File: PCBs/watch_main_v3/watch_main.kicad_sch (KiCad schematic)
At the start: 1 part, among them U101 Watch_Outline_V2

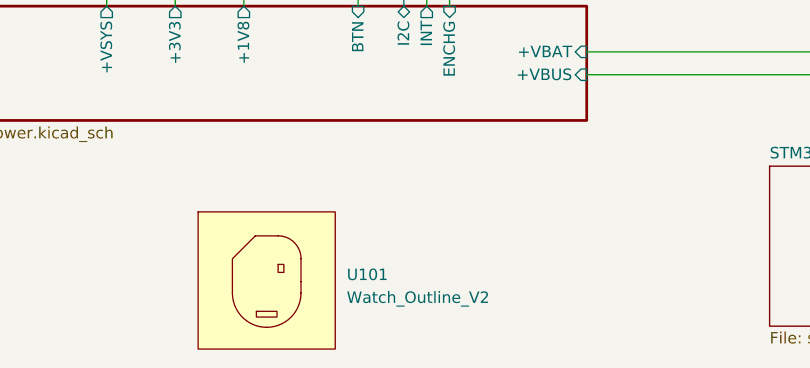
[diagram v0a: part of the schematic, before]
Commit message: watch_main_v3 updates
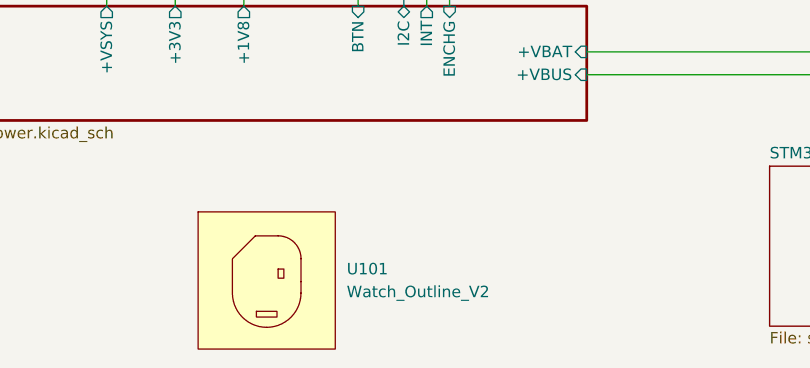
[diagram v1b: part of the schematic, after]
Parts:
- U101: footprint watch_footprints:Watch Outline V2 -> watch_footprints:Watch Outline V3; symbol watch_symbols_lib:Watch_Outline_V2 -> watch_symbols_lib:Watch_Outline_V3
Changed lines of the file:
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@@
     )
   )
-  (symbol (lib_id "watch_symbols_lib:Watch_Outline_V2") (at 73.66 177.8 0) (unit 1)
+  (symbol (lib_id "watch_symbols_lib:Watch_Outline_V3") (at 73.66 177.8 0) (unit 1)
     (in_bom no) (on_board yes) (dnp no) (fields_autoplaced)
-    (property "Reference" "U101" (at 82.55 177.165 0)
+    (property "Reference" "U101" (at 82.55 176.53 0)
       (effects (font (size 1.27 1.27)) (justify left))
     )
-    (property "Value" "Watch_Outline_V2" (at 82.55 179.705 0)
+    (property "Value" "Watch_Outline_V2" (at 82.55 179.07 0)
       (effects (font (size 1.27 1.27)) (justify left))
     )
-    (property "Footprint" "watch_footprints:Watch Outline V2" (at 73.66 187.96 0)
+    (property "Footprint" "watch_footprints:Watch Outline V3" (at 73.66 187.96 0)
       (effects (font (size 1.27 1.27)) hide)
     )
